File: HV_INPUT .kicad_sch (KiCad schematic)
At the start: 6 parts, among them J1 Screw_Terminal_01x03

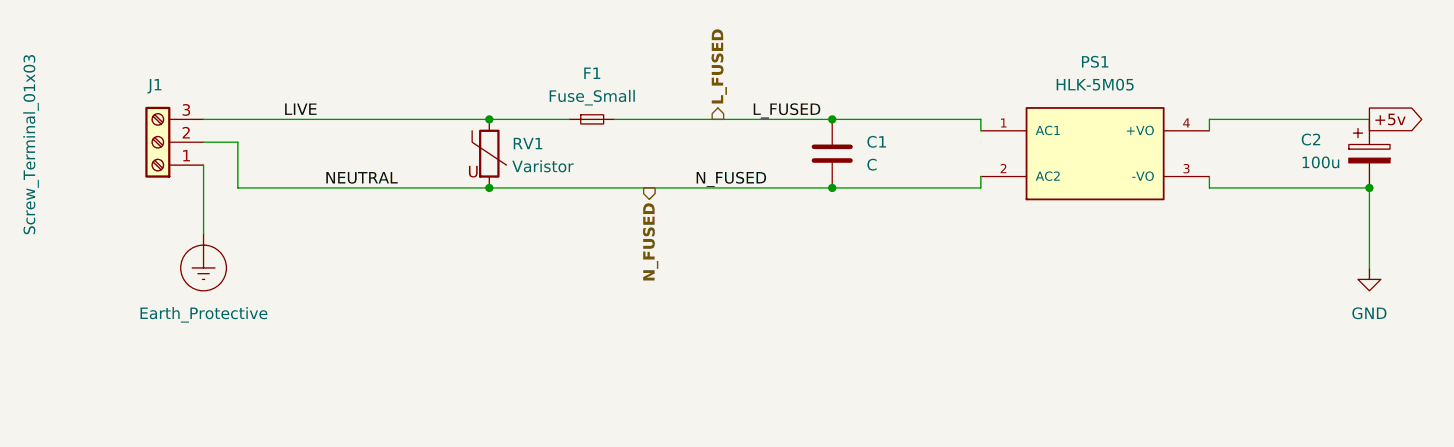
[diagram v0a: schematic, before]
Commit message: Update KiCad project files
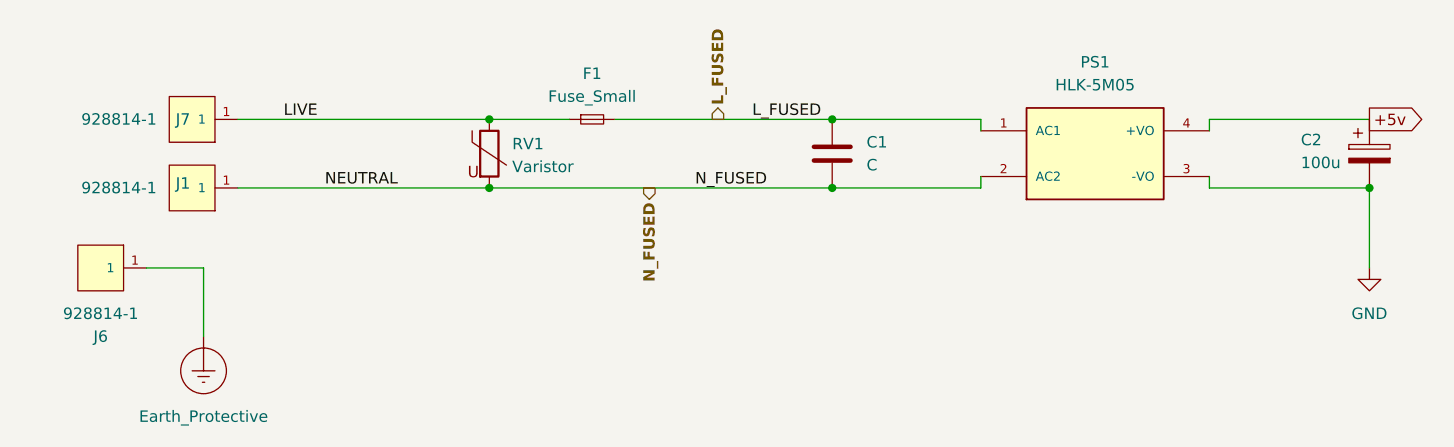
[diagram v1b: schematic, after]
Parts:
- removed J1: Screw_Terminal_01x03, symbol Connector:Screw_Terminal_01x03
- added J1, J6, J7: 928814-1, 6.3mm spade:TE_928814-1, symbol 6.3mm spade:928814-1
- PS1: footprint HLK-5M05:CONV_HLK-5M05 -> HLK_5M05:CONV_HLK-5M05
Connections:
- net Earth_Protective: now also J6.1
- net LIVE: now also J7.1
- net N_FUSED: now also J1.1
